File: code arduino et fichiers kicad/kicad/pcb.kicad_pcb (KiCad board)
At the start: 4 copper layers, 53.3 x 101.6 mm, 32 parts, among them J1 Screw_Terminal_01x04, J2 Screw_Terminal_01x04, J3 Screw_Terminal_01x02, U1 LMC6482, U2 LMC6482, U3 LMC6482

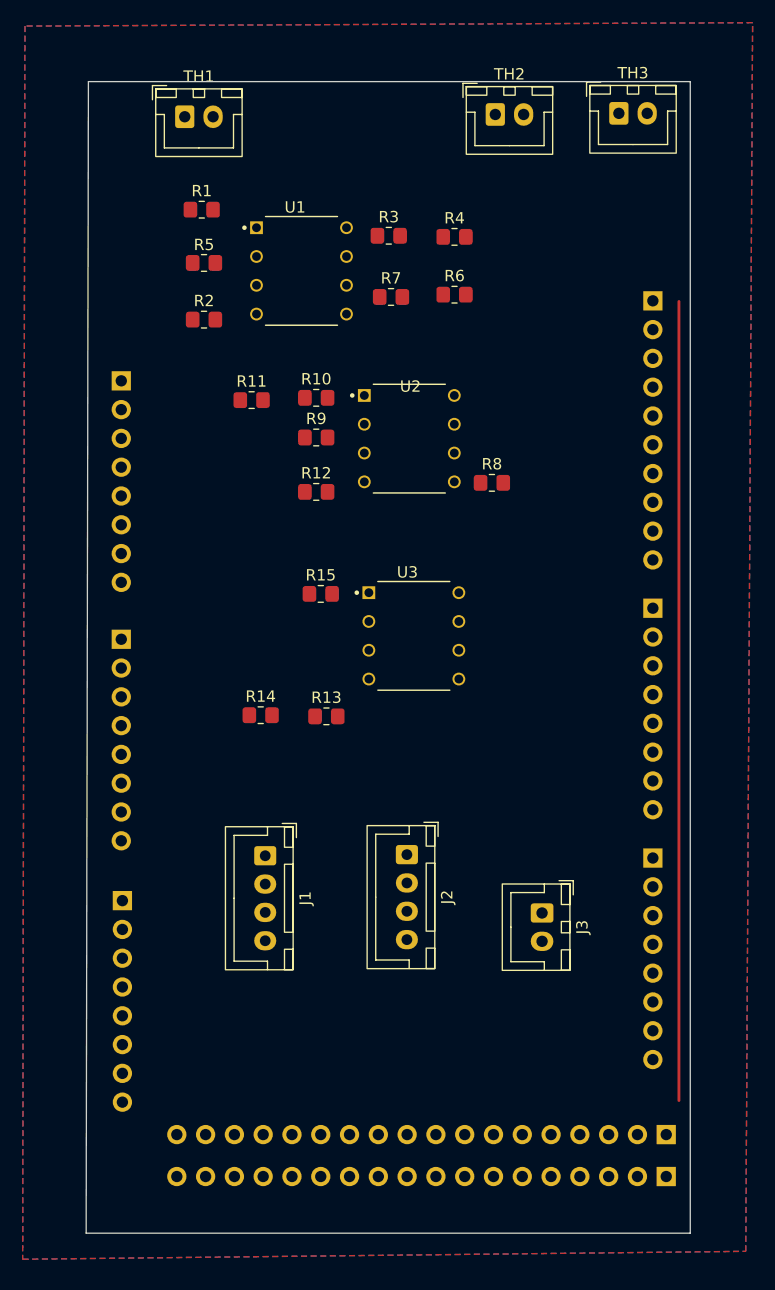
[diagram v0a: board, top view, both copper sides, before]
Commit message: procrastination pendant optique
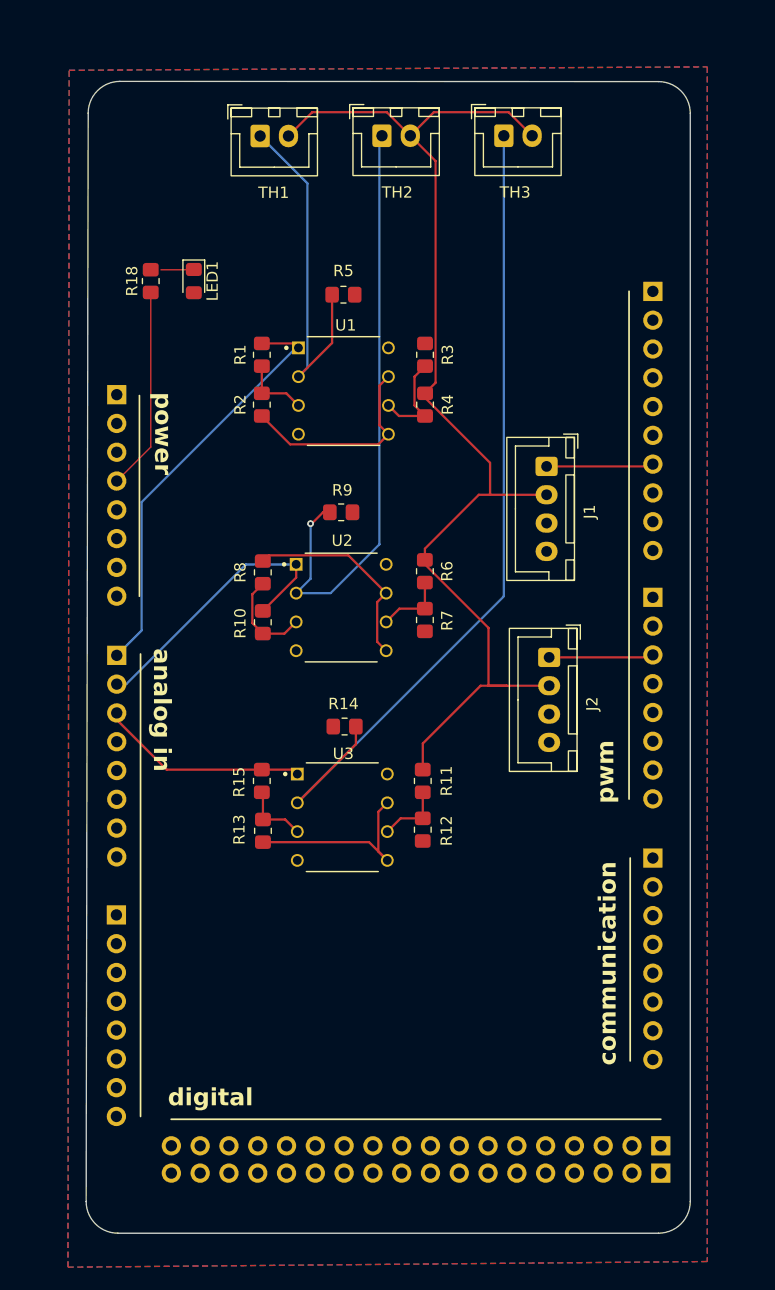
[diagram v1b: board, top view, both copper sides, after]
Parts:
- removed J3: Screw_Terminal_01x02, Connector_JST:JST_XH_B2B-XH-A_1x02_P2.50mm_Vertical
- added LED1: LED_LEDCHIP-LED0805, LED_SMD:LED_0805_2012Metric_Pad1.15x1.40mm_HandSolder, F.Cu at (78.9, 57.8)
- added R18: 560, Resistor_SMD:R_0805_2012Metric_Pad1.20x1.40mm_HandSolder, F.Cu at (75.1, 57.8)
- moved J1 42.4 mm to (110.0, 74.2)
- moved R11 36.8 mm to (99.1, 101.9), turned to -90 degrees
- moved R12 31.2 mm to (99.1, 106.2), turned to 90 degrees
- moved R7 28.7 mm to (99.3, 87.7), turned to 90 degrees
- moved R6 24.5 mm to (99.3, 83.4), turned to -90 degrees
- moved R8 21.7 mm to (85.0, 83.5), turned to -90 degrees
- moved J2 21.5 mm to (110.2, 91.0)
- moved R10 20.4 mm to (85.0, 87.9), turned to 90 degrees
- moved R15 17.3 mm to (84.9, 101.9), turned to 90 degrees
- moved U3 17.2 mm to (92.0, 105.1)
- moved U2 16.1 mm to (91.9, 86.6)
- moved R4 15.0 mm to (99.3, 68.7), turned to -90 degrees
- moved R1 13.9 mm to (84.9, 64.3), turned to 90 degrees
- moved R5 12.6 mm to (92.1, 59.0), turned to 180 degrees
- moved R13 11.5 mm to (85.0, 106.3), turned to 90 degrees
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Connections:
- power2 pad 4: unconnected-(power2-Pin_4-Pad4) -> +3.3V
- power2 pad 5: unconnected-(power2-Pin_5-Pad5) -> 5V
- power2 pad 7: unconnected-(power2-Pin_7-Pad7) -> GND
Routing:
- net +5V: track 0.00 -> 104.6 mm
- net Net-(U3A--): track 0.00 -> 75.3 mm
- net Net-(U2A--): track 0.00 -> 54.0 mm, vias 0 -> 1
- net T1 sortie: track 0.00 -> 37.3 mm
- net Net-(U1A--): track 0.00 -> 31.7 mm
- net T2 sortie: track 0.00 -> 25.5 mm
- net T3 sortie: track 0.00 -> 18.5 mm
- net Net-(U1B-+): track 0.00 -> 18.3 mm
- net Net-(U2B-+): track 0.00 -> 18.2 mm
- net +3.3V: track 0.00 -> 17.9 mm
- net Net-(U3B-+): track 0.00 -> 17.4 mm
- net pwmgauche: track 0.00 -> 9.46 mm
- net pwmdroite: track 0.00 -> 9.24 mm
- net Net-(U1B--): track 0.00 -> 8.78 mm
- net Net-(U2A-+): track 0.00 -> 8.54 mm
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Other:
- outline, holes or cut-outs redrawn
- board text added: "R14"
- board text added: "analog in"
- board text added: "communication"
- board text added: "digital"
- board text added: "power"
- board text added: "pwm"
